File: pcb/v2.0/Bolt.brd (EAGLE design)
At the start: 63.6 x 48.9 mm, 45 parts, among them J1 10118194-0001LF, Q1 XT60_YELLOW, Q2 MMSS8050-H-TP, Q3 MMSS8050-H-TP, U1 FT231XS-R, U2 ESP32-WROOM-32D, U3 LM1117DT-3.3/NOPB

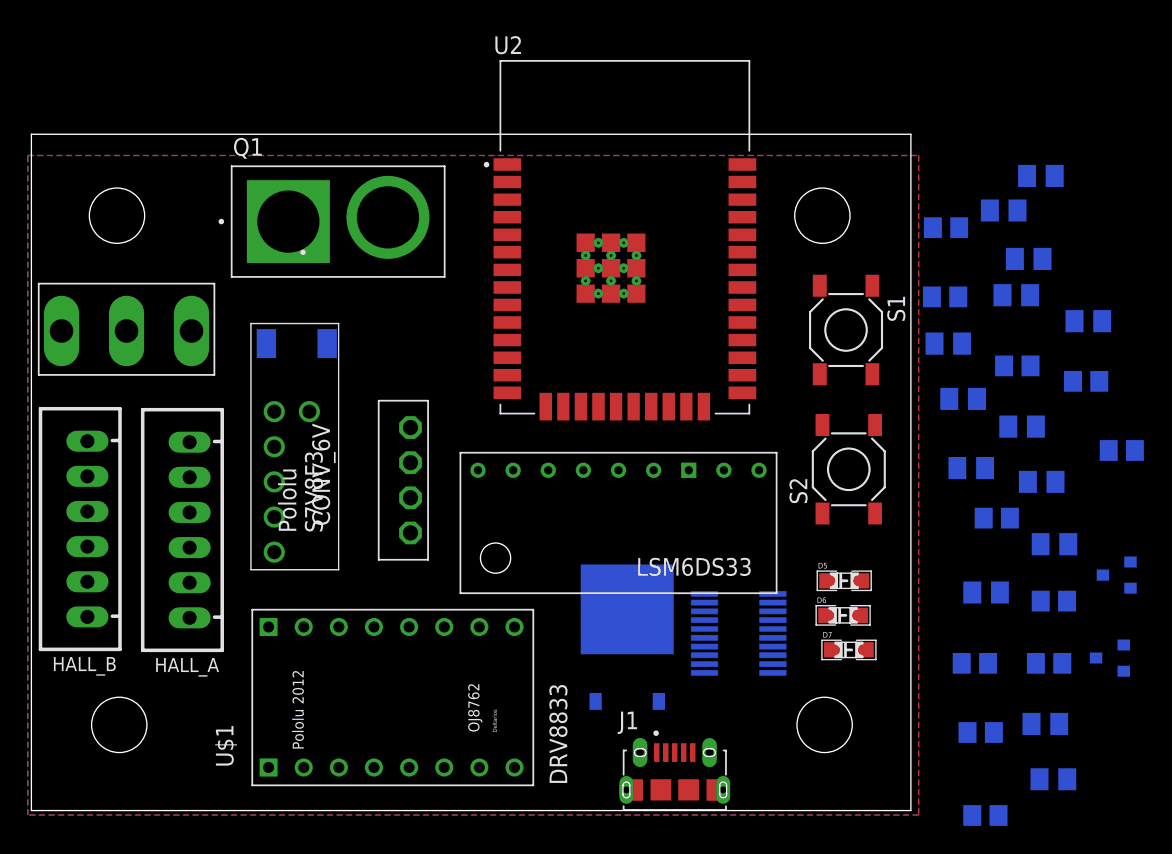
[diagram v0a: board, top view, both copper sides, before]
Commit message: Routes except VCC
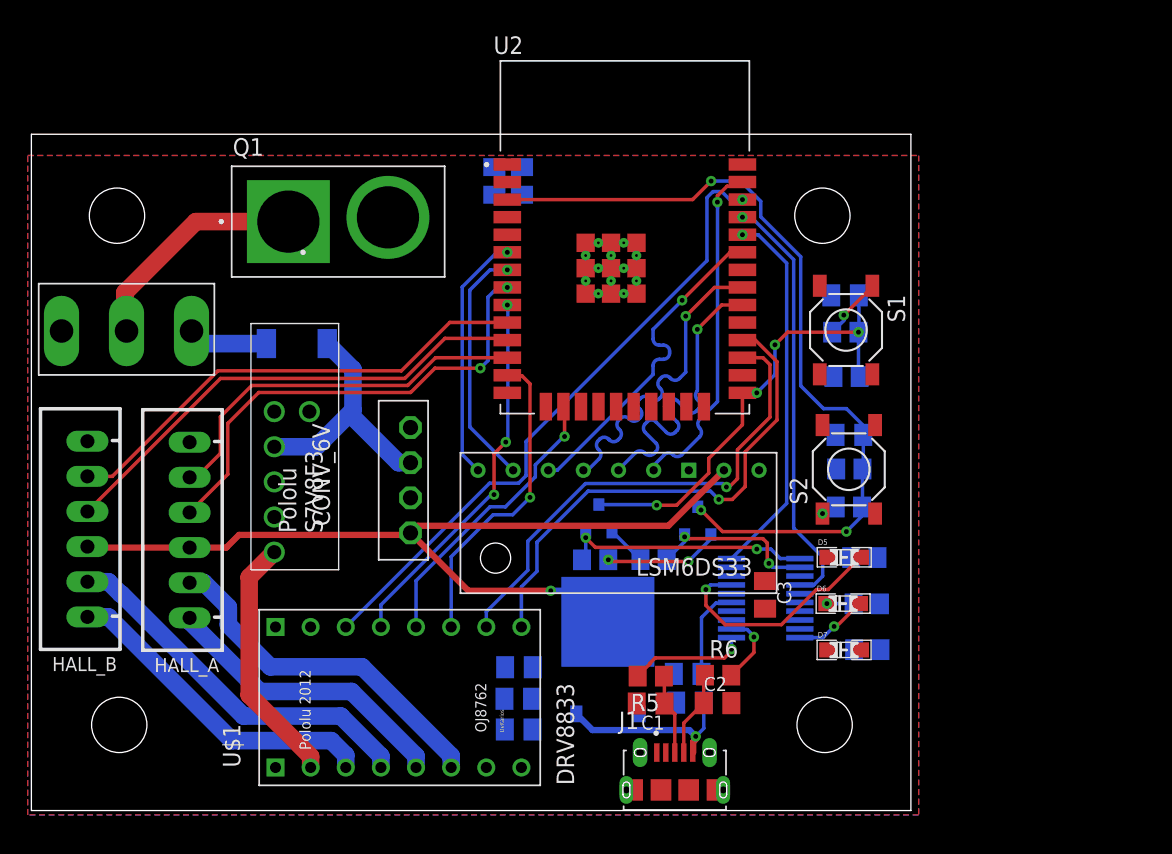
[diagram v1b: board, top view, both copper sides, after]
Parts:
- removed C6: 10uF, rcl:C0805K
- removed C7: 0.1uF, rcl:C0805K
- moved C13 49.8 mm to (51.0, 26.1)
- moved C8 46.6 mm to (51.2, 63.6), turned to 90 degrees
- moved C10 45.8 mm to (63.4, 25.9)
- moved C12 40.1 mm to (51.0, 28.4)
- moved R9 37.8 mm to (56.5, 36.2)
- moved Q2 37.7 mm to (56.8, 39.2), turned to 90 degrees
- moved C9 37.4 mm to (49.2, 63.6), turned to 90 degrees
- moved C2 36.6 mm to (65.4, 25.8), flipped to the top
- moved R6 36.3 mm to (65.4, 27.8), flipped to the top
- moved C14 35.2 mm to (51.0, 23.9)
- moved R5 34.7 mm to (60.5, 27.8), flipped to the top, turned to 180 degrees
- moved C1 33.5 mm to (60.5, 25.8), flipped to the top, turned to 180 degrees
- moved Q3 31.4 mm to (63.9, 39.0), turned to 90 degrees
- moved R10 30.3 mm to (60.7, 36.2)
- moved C11 25.3 mm to (63.2, 27.9)
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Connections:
- removed net USB_5V: C6.1, C7.1
- net GND: no longer C6.2, C7.2
- net HALL_B1: now also U2.11; no longer U2.10
- net HALL_B2: now also U2.10; no longer U2.11
- net MA_1: now also U$1.OA2; no longer U$1.OA1
- net MA_2: now also U$1.OA1; no longer U$1.OA2
- net PWM_IN_A1: now also U$1.INA2; no longer U$1.INA1
- net PWM_IN_A2: now also U$1.INA1; no longer U$1.INA2
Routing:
- net VCC: track 0.00 -> 64.7 mm, vias 0 -> 1
- net EN: track 0.00 -> 59.4 mm, vias 0 -> 3
- net PWM_IN_B1: track 0.00 -> 46.1 mm, vias 0 -> 1
- net DRV_FAULT: track 0.00 -> 36.9 mm, vias 0 -> 1
- net DRV_SLEEP: track 0.00 -> 36.1 mm, vias 0 -> 1
- net HALL_B1: track 0.00 -> 35.6 mm
- net HALL_B2: track 0.00 -> 35.0 mm
- net HALL_A1: track 0.00 -> 34.6 mm, vias 0 -> 2
- net IO0: track 0.00 -> 33.1 mm, vias 0 -> 4
- net TXD0: track 0.00 -> 30.6 mm, vias 0 -> 1
- net HALL_A2: track 0.00 -> 28.1 mm
- net MB_2: track 0.00 -> 27.3 mm
- net PWM_IN_B2: track 0.00 -> 27.2 mm, vias 0 -> 3
- net RXD0: track 0.00 -> 27.1 mm, vias 0 -> 1
- net MA_2: track 0.00 -> 25.7 mm
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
